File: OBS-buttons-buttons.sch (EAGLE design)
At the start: 23 parts

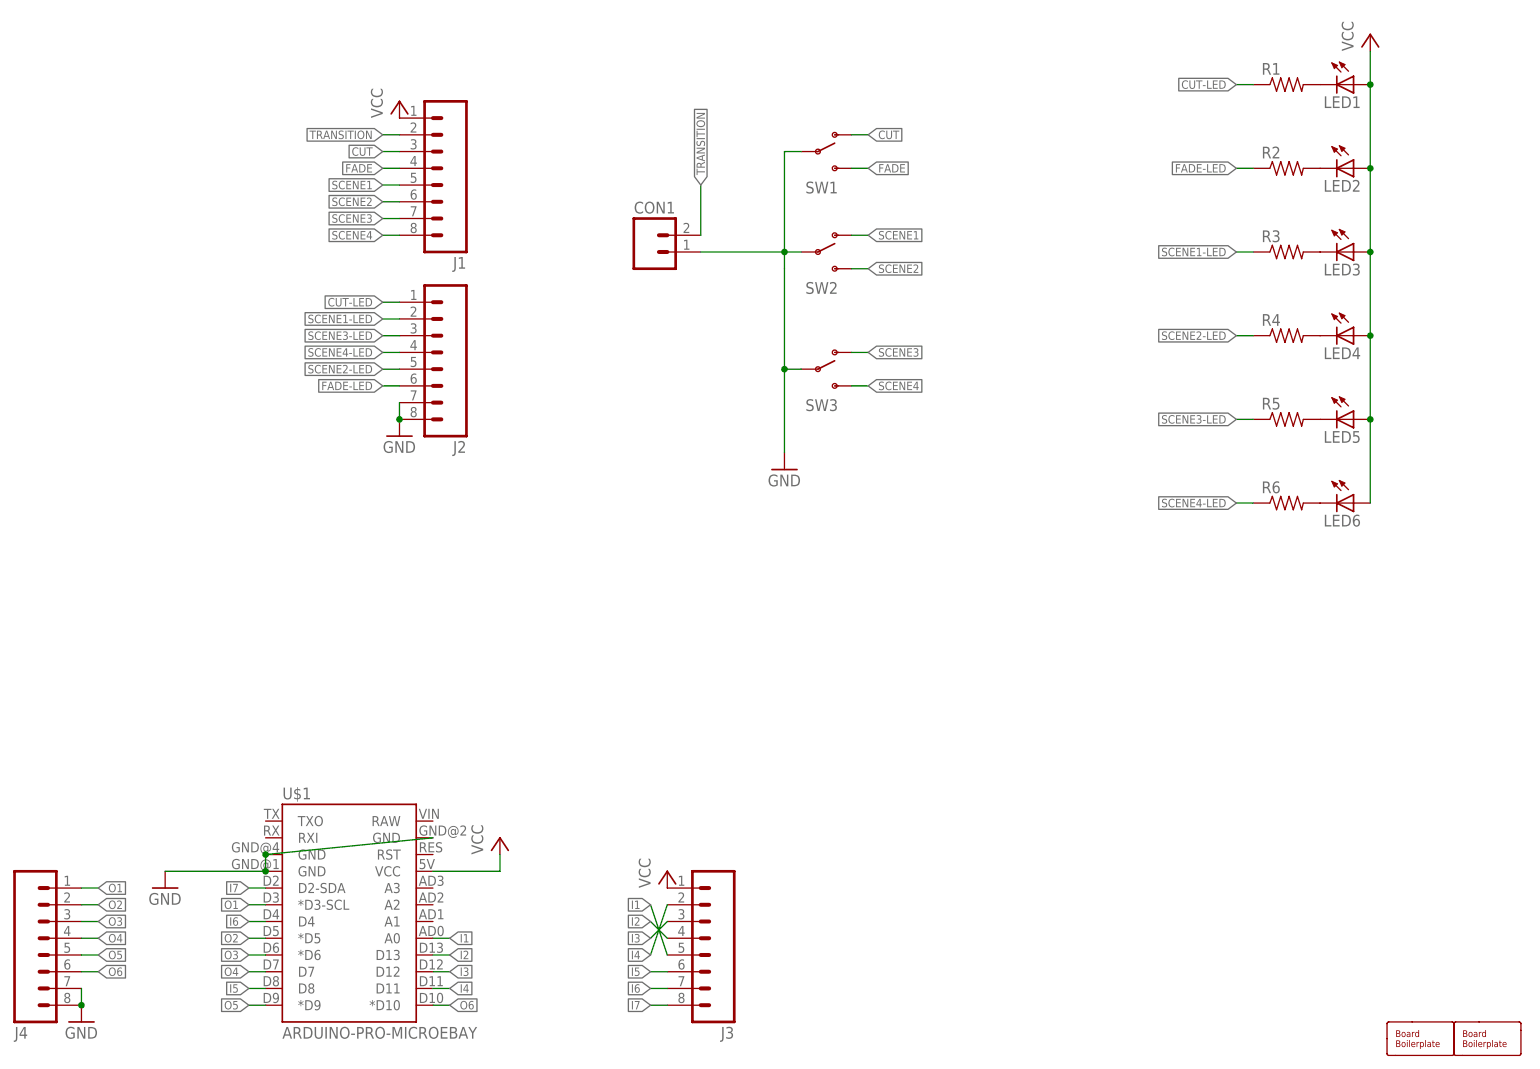
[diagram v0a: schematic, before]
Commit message: initial prototype
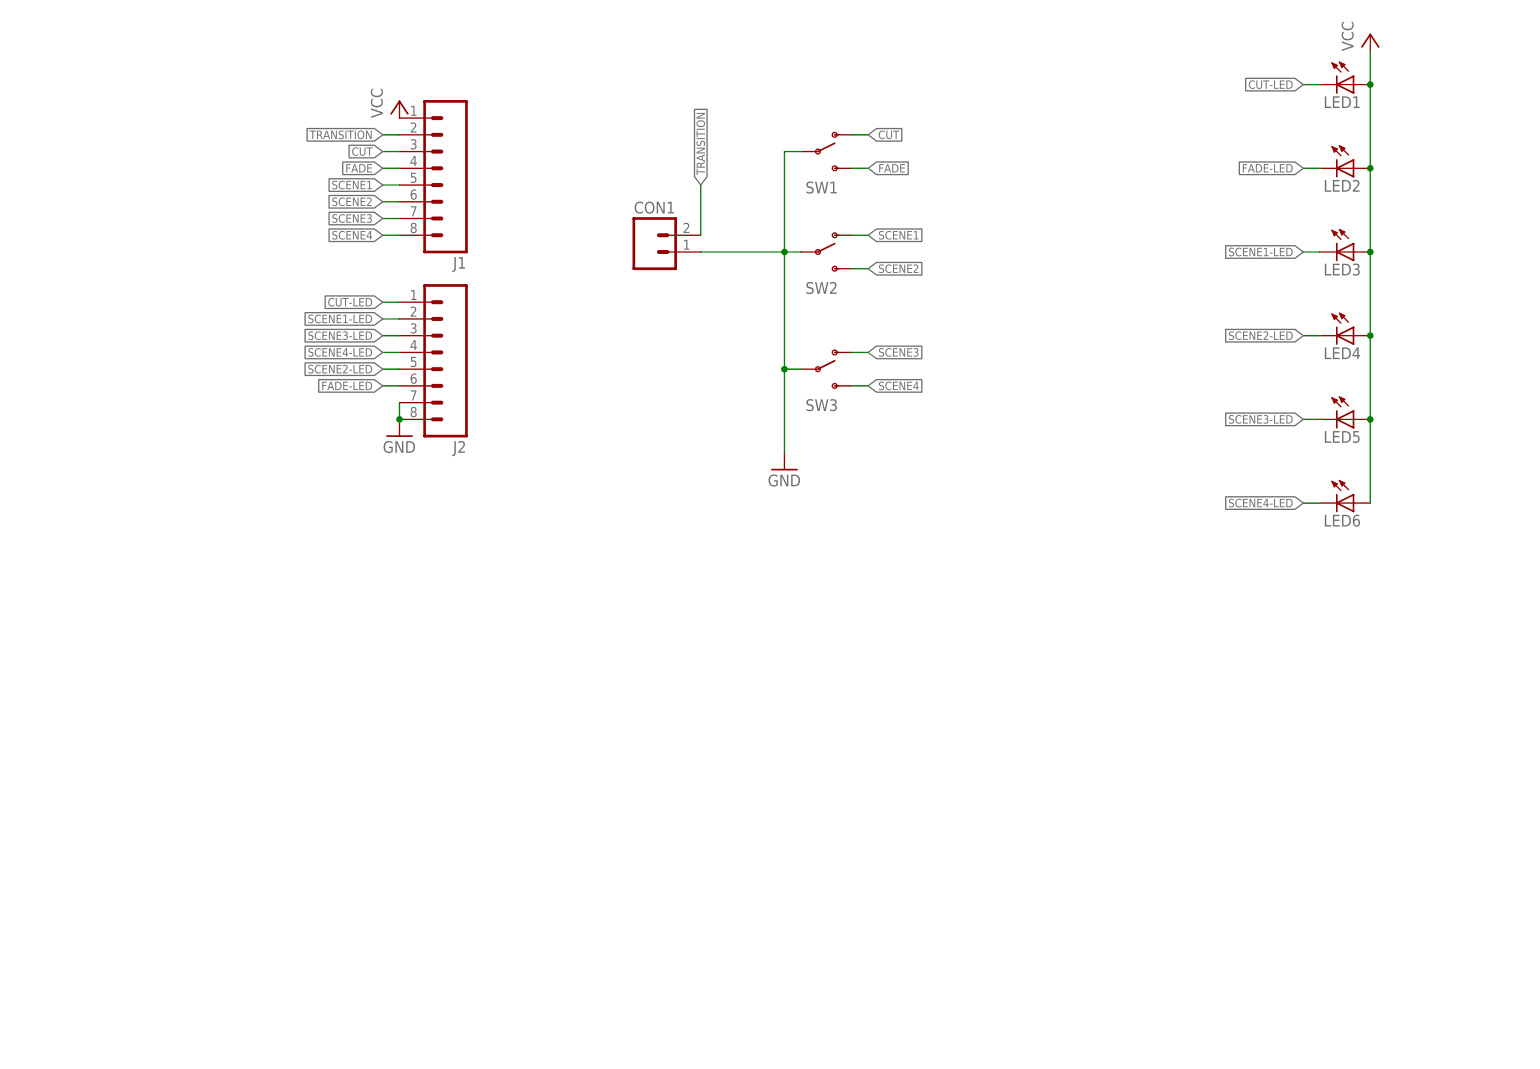
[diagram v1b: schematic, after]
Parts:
- removed BOARD1, BOARD2: (no value), SPCoast:BOARD100X50-NOHOLES
- removed J3, J4: (no value), SPCoast:CONNECTOR-M08LOCK
- removed R1, R2, R3, R4, R5, R6: (no value), SPCoast:RPTH04
- removed U$1: ARDUINO-PRO-MICROEBAY, SPCoast:ARDUINO-PRO-MICROEBAY
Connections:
- removed net I1: J3.5, U$1.A0
- removed net I2: J3.4, U$1.D13
- removed net I3: J3.3, U$1.D12
- removed net I4: J3.2, U$1.D11
- removed net I5: J3.6, U$1.D8
- removed net I6: J3.7, U$1.D4
- removed net I7: J3.8, U$1.D2-SDA
- removed net N$1: LED1.C, R1.2
- removed net N$2: LED2.C, R2.2
- removed net N$3: LED3.C, R3.2
- removed net N$4: LED4.C, R4.2
- removed net N$5: LED5.C, R5.2
- removed net N$6: LED6.C, R6.2
- removed net O1: J4.1, U$1.*D3-SCL
- removed net O2: J4.2, U$1.*D5
- removed net O3: J4.3, U$1.*D6
- removed net O4: J4.4, U$1.D7
- removed net O5: J4.5, U$1.*D9
- removed net O6: J4.6, U$1.*D10
- net CUT-LED: now also LED1.C; no longer R1.1
- net FADE-LED: now also LED2.C; no longer R2.1
- net GND: no longer J4.7, J4.8, U$1.GND, U$1.GND@2, U$1.GND@3
- net SCENE1-LED: now also LED3.C; no longer R3.1
- net SCENE2-LED: now also LED4.C; no longer R4.1
- net SCENE3-LED: now also LED5.C; no longer R5.1
- net SCENE4-LED: now also LED6.C; no longer R6.1
- net VCC: no longer J3.1, U$1.VCC
